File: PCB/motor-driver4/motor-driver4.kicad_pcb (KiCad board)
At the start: 2 copper layers, 100 x 100 mm, 57 parts, among them J1 Motor Power, J2 Input Logic, M1 Motor_DC, M2 Motor_DC, Q1 Q_NMOS_GDS, Q2 Q_NMOS_GDS, Q3 Q_NMOS_GDS, Q4 Q_NMOS_GDS, Q5 Q_NMOS_GDS, Q6 Q_NMOS_GDS, Q7 Q_NMOS_GDS, Q8 Q_NMOS_GDS, U1 IR2302, U2 IR2302, U3 IR2302, U4 IR2302

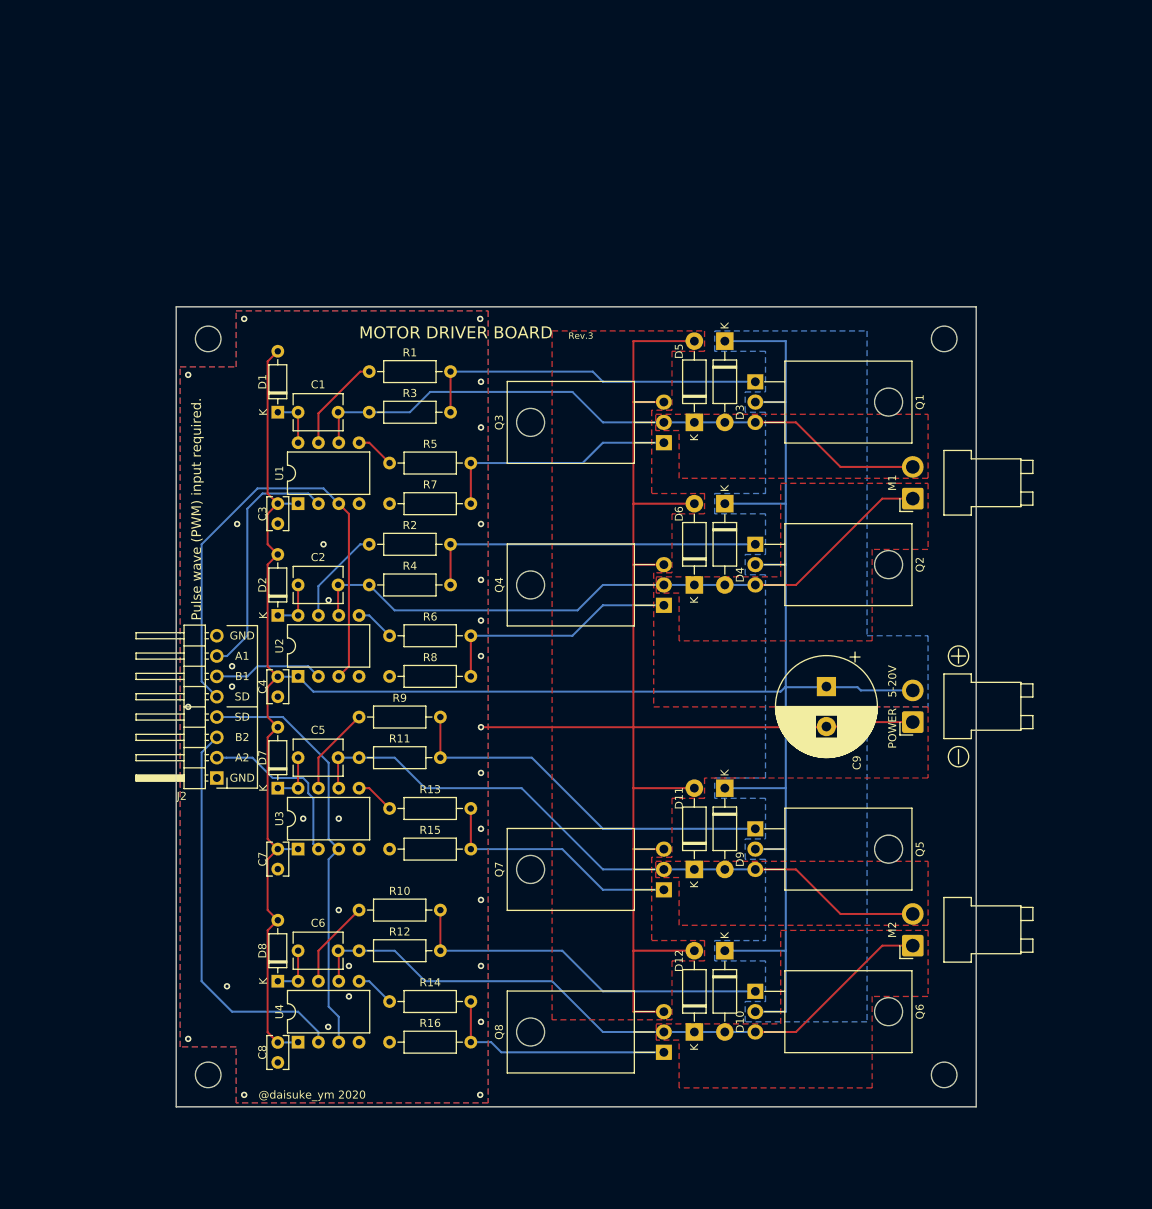
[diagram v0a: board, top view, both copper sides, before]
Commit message: ほぼ完成
git-svn-id: https://shiro-home.ddns.net/svn/project/motor-driver/trunk@12 73406841-da20-4056-b287-c5b29fcc9b8e
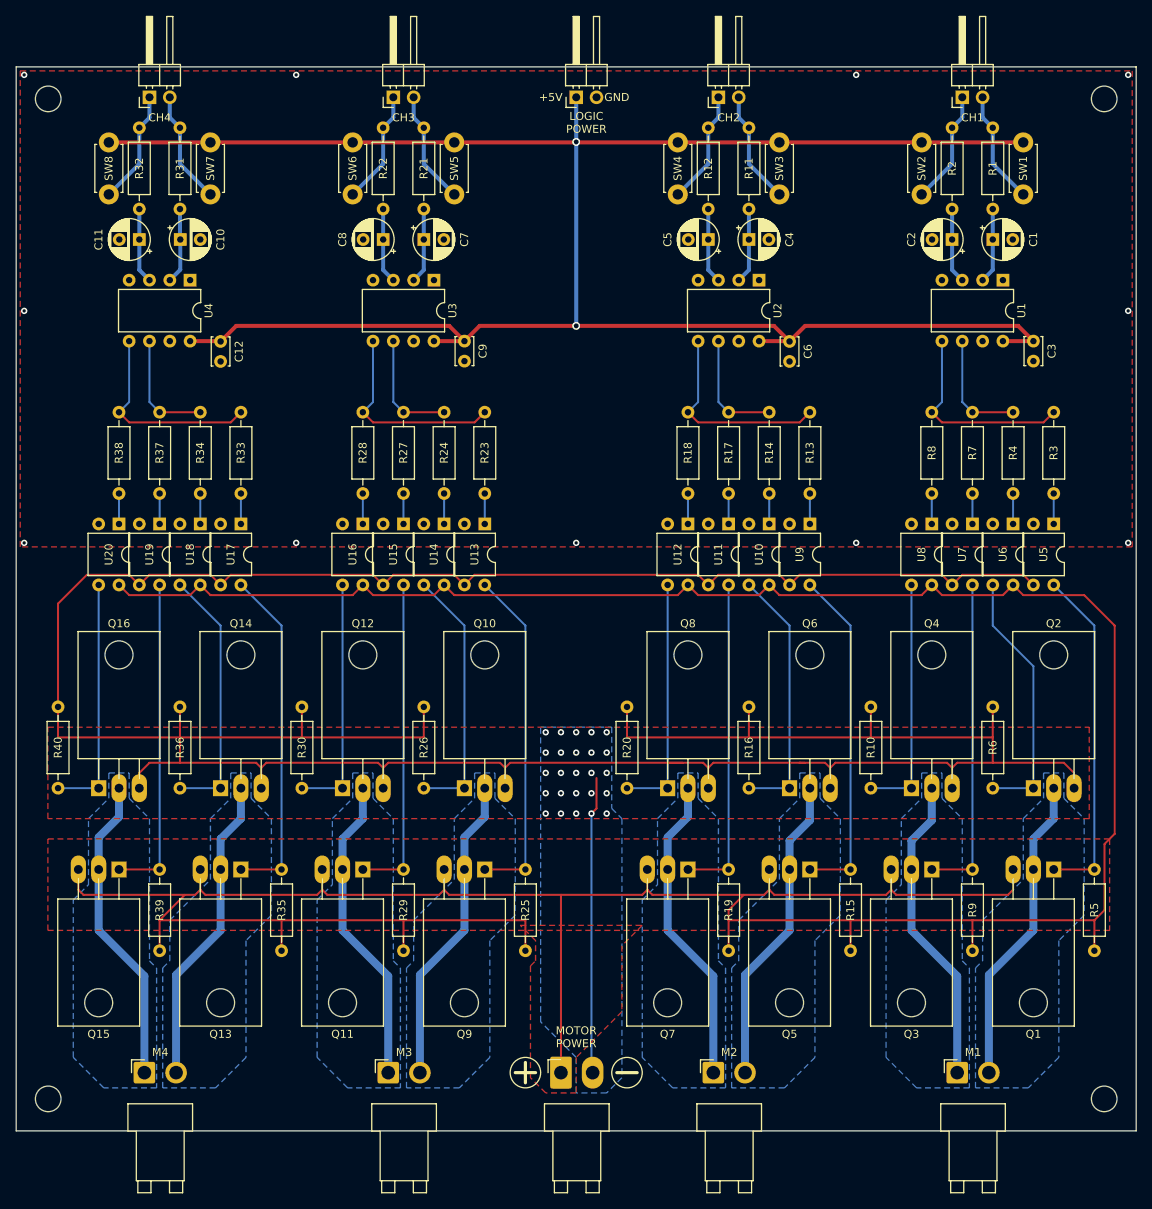
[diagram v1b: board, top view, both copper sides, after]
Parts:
- removed D1, D2, D7, D8: 1N4148, Diode_THT:D_DO-35_SOD27_P7.62mm_Horizontal
- removed D10, D11, D12, D3, D4, D5, D6, D9: 1N4007, Diode_THT:D_DO-41_SOD81_P10.16mm_Horizontal
- added C10: 10u, Capacitor_THT:CP_Radial_D5.0mm_P2.50mm, F.Cu at (100.5, 41.6)
- added C11: 10u, Capacitor_THT:CP_Radial_D5.0mm_P2.50mm, F.Cu at (95.4, 41.6)
- added C12: 0.1u, Capacitor_THT:C_Disc_D3.4mm_W2.1mm_P2.50mm, F.Cu at (105.5, 54.3)
- added J3: Input Ch1, Connector_PinHeader_2.54mm:PinHeader_1x02_P2.54mm_Horizontal, F.Cu at (198.3, 23.8)
- added J4: Input Ch2, Connector_PinHeader_2.54mm:PinHeader_1x02_P2.54mm_Horizontal, F.Cu at (167.8, 23.8)
- added J5: Input Ch3, Connector_PinHeader_2.54mm:PinHeader_1x02_P2.54mm_Horizontal, F.Cu at (127.1, 23.8)
- added J6: Input Ch4, Connector_PinHeader_2.54mm:PinHeader_1x02_P2.54mm_Horizontal, F.Cu at (96.7, 23.8)
- added M3: Motor_DC, Connector_JST:JST_VH_B2PS-VH_1x02_P3.96mm_Horizontal, F.Cu at (126.5, 145.7)
- added M4: Motor_DC, Connector_JST:JST_VH_B2PS-VH_1x02_P3.96mm_Horizontal, F.Cu at (96.0, 145.7)
- added Q10: Q_NMOS_GDS, Package_TO_SOT_THT:TO-220-3_Horizontal_TabDown, F.Cu at (136.0, 110.2)
- added Q11: Q_PMOS_GDS, Package_TO_SOT_THT:TO-220-3_Horizontal_TabDown, F.Cu at (123.3, 120.3)
- added Q12: Q_NMOS_GDS, Package_TO_SOT_THT:TO-220-3_Horizontal_TabDown, F.Cu at (120.8, 110.2)
- added Q13: Q_PMOS_GDS, Package_TO_SOT_THT:TO-220-3_Horizontal_TabDown, F.Cu at (108.1, 120.3)
- added Q14: Q_NMOS_GDS, Package_TO_SOT_THT:TO-220-3_Horizontal_TabDown, F.Cu at (105.5, 110.2)
- added Q15: Q_PMOS_GDS, Package_TO_SOT_THT:TO-220-3_Horizontal_TabDown, F.Cu at (92.8, 120.3)
- added Q16: Q_NMOS_GDS, Package_TO_SOT_THT:TO-220-3_Horizontal_TabDown, F.Cu at (90.3, 110.2)
- added Q9: Q_PMOS_GDS, Package_TO_SOT_THT:TO-220-3_Horizontal_TabDown, F.Cu at (138.6, 120.3)
- added R17: 330, Resistor_THT:R_Axial_DIN0207_L6.3mm_D2.5mm_P10.16mm_Horizontal, F.Cu at (169.1, 63.2)
- added R18: 330, Resistor_THT:R_Axial_DIN0207_L6.3mm_D2.5mm_P10.16mm_Horizontal, F.Cu at (164.0, 63.2)
- added R19: 2k2, Resistor_THT:R_Axial_DIN0207_L6.3mm_D2.5mm_P10.16mm_Horizontal, F.Cu at (169.1, 120.3)
- added R20: 2k2, Resistor_THT:R_Axial_DIN0207_L6.3mm_D2.5mm_P10.16mm_Horizontal, F.Cu at (156.3, 100.0)
- added R21: 4k7, Resistor_THT:R_Axial_DIN0207_L6.3mm_D2.5mm_P10.16mm_Horizontal, F.Cu at (130.9, 27.6)
- added R22: 4k7, Resistor_THT:R_Axial_DIN0207_L6.3mm_D2.5mm_P10.16mm_Horizontal, F.Cu at (125.9, 27.6)
- added R23: 330, Resistor_THT:R_Axial_DIN0207_L6.3mm_D2.5mm_P10.16mm_Horizontal, F.Cu at (138.6, 63.2)
- added R24: 330, Resistor_THT:R_Axial_DIN0207_L6.3mm_D2.5mm_P10.16mm_Horizontal, F.Cu at (133.5, 63.2)
- added R25: 2k2, Resistor_THT:R_Axial_DIN0207_L6.3mm_D2.5mm_P10.16mm_Horizontal, F.Cu at (143.7, 120.3)
- added R26: 2k2, Resistor_THT:R_Axial_DIN0207_L6.3mm_D2.5mm_P10.16mm_Horizontal, F.Cu at (130.9, 100.0)
- added R27: 330, Resistor_THT:R_Axial_DIN0207_L6.3mm_D2.5mm_P10.16mm_Horizontal, F.Cu at (128.4, 63.2)
- added R28: 330, Resistor_THT:R_Axial_DIN0207_L6.3mm_D2.5mm_P10.16mm_Horizontal, F.Cu at (123.3, 63.2)
- added R29: 2k2, Resistor_THT:R_Axial_DIN0207_L6.3mm_D2.5mm_P10.16mm_Horizontal, F.Cu at (128.4, 120.3)
- added R30: 2k2, Resistor_THT:R_Axial_DIN0207_L6.3mm_D2.5mm_P10.16mm_Horizontal, F.Cu at (115.7, 100.0)
- added R31: 4k7, Resistor_THT:R_Axial_DIN0207_L6.3mm_D2.5mm_P10.16mm_Horizontal, F.Cu at (100.5, 27.6)
- added R32: 4k7, Resistor_THT:R_Axial_DIN0207_L6.3mm_D2.5mm_P10.16mm_Horizontal, F.Cu at (95.4, 27.6)
- added R33: 330, Resistor_THT:R_Axial_DIN0207_L6.3mm_D2.5mm_P10.16mm_Horizontal, F.Cu at (108.1, 63.2)
- added R34: 330, Resistor_THT:R_Axial_DIN0207_L6.3mm_D2.5mm_P10.16mm_Horizontal, F.Cu at (103.0, 63.2)
- added R35: 2k2, Resistor_THT:R_Axial_DIN0207_L6.3mm_D2.5mm_P10.16mm_Horizontal, F.Cu at (113.2, 120.3)
- added R36: 2k2, Resistor_THT:R_Axial_DIN0207_L6.3mm_D2.5mm_P10.16mm_Horizontal, F.Cu at (100.5, 100.0)
- added R37: 330, Resistor_THT:R_Axial_DIN0207_L6.3mm_D2.5mm_P10.16mm_Horizontal, F.Cu at (97.9, 63.2)
- added R38: 330, Resistor_THT:R_Axial_DIN0207_L6.3mm_D2.5mm_P10.16mm_Horizontal, F.Cu at (92.8, 63.2)
- added R39: 2k2, Resistor_THT:R_Axial_DIN0207_L6.3mm_D2.5mm_P10.16mm_Horizontal, F.Cu at (97.9, 120.3)
- added R40: 2k2, Resistor_THT:R_Axial_DIN0207_L6.3mm_D2.5mm_P10.16mm_Horizontal, F.Cu at (85.2, 100.0)
- added SW1: SW_Push, MyLib:TactSW_TVBP06_3.5x6.0-ThroughHole, F.Cu at (205.9, 32.7)
- added SW2: SW_Push, MyLib:TactSW_TVBP06_3.5x6.0-ThroughHole, F.Cu at (193.2, 32.7)
- added SW3: SW_Push, MyLib:TactSW_TVBP06_3.5x6.0-ThroughHole, F.Cu at (175.4, 32.7)
- added SW4: SW_Push, MyLib:TactSW_TVBP06_3.5x6.0-ThroughHole, F.Cu at (162.7, 32.7)
- added SW5: SW_Push, MyLib:TactSW_TVBP06_3.5x6.0-ThroughHole, F.Cu at (134.8, 32.7)
- added SW6: SW_Push, MyLib:TactSW_TVBP06_3.5x6.0-ThroughHole, F.Cu at (122.1, 32.7)
- added SW7: SW_Push, MyLib:TactSW_TVBP06_3.5x6.0-ThroughHole, F.Cu at (104.3, 32.7)
- added SW8: SW_Push, MyLib:TactSW_TVBP06_3.5x6.0-ThroughHole, F.Cu at (91.6, 32.7)
- added U10: TLP785, Package_DIP:DIP-4_W7.62mm, F.Cu at (174.1, 77.1)
- added U11: TLP785, Package_DIP:DIP-4_W7.62mm, F.Cu at (169.1, 77.1)
- added U12: TLP785, Package_DIP:DIP-4_W7.62mm, F.Cu at (164.0, 77.1)
- added U13: TLP785, Package_DIP:DIP-4_W7.62mm, F.Cu at (138.6, 77.1)
- added U14: TLP785, Package_DIP:DIP-4_W7.62mm, F.Cu at (133.5, 77.1)
- added U15: TLP785, Package_DIP:DIP-4_W7.62mm, F.Cu at (128.4, 77.1)
- added U16: TLP785, Package_DIP:DIP-4_W7.62mm, F.Cu at (123.3, 77.1)
- added U17: TLP785, Package_DIP:DIP-4_W7.62mm, F.Cu at (108.1, 77.1)
- added U18: TLP785, Package_DIP:DIP-4_W7.62mm, F.Cu at (103.0, 77.1)
- added U19: TLP785, Package_DIP:DIP-4_W7.62mm, F.Cu at (97.9, 77.1)
- added U20: TLP785, Package_DIP:DIP-4_W7.62mm, F.Cu at (92.8, 77.1)
- added U5: TLP785, Package_DIP:DIP-4_W7.62mm, F.Cu at (209.7, 77.1)
- added U6: TLP785, Package_DIP:DIP-4_W7.62mm, F.Cu at (204.6, 77.1)
- added U7: TLP785, Package_DIP:DIP-4_W7.62mm, F.Cu at (199.5, 77.1)
- added U8: TLP785, Package_DIP:DIP-4_W7.62mm, F.Cu at (194.4, 77.1)
- added U9: TLP785, Package_DIP:DIP-4_W7.62mm, F.Cu at (179.2, 77.1)
- C1, C2, C5: footprint Capacitor_THT:C_Disc_D6.0mm_W4.4mm_P5.00mm -> Capacitor_THT:CP_Radial_D5.0mm_P2.50mm
- C3: footprint Capacitor_THT:C_Rect_L4.0mm_W2.5mm_P2.50mm -> Capacitor_THT:C_Disc_D3.4mm_W2.1mm_P2.50mm
- C4, C7, C8: value 0.1u -> 10u; footprint Capacitor_THT:C_Rect_L4.0mm_W2.5mm_P2.50mm -> Capacitor_THT:CP_Radial_D5.0mm_P2.50mm
- C6: value 10u -> 0.1u; footprint Capacitor_THT:C_Disc_D6.0mm_W4.4mm_P5.00mm -> Capacitor_THT:C_Disc_D3.4mm_W2.1mm_P2.50mm
- C9: value 470u 50V -> 0.1u; footprint Capacitor_THT:CP_Radial_D12.5mm_P5.00mm -> Capacitor_THT:C_Disc_D3.4mm_W2.1mm_P2.50mm
- J2: value Input Logic -> Logic Power; footprint Connector_PinHeader_2.54mm:PinHeader_1x08_P2.54mm_Horizontal -> Connector_PinHeader_2.54mm:PinHeader_1x02_P2.54mm_Horizontal
- Q1, Q3, Q5, Q7: value Q_NMOS_GDS -> Q_PMOS_GDS
- R1, R11, R12, R2: value 47k -> 4k7
- R10, R15, R16, R5, R6, R9: value 47k -> 2k2
- R13, R14, R3, R4, R7, R8: value 47k -> 330
- U1, U2, U3, U4: value IR2302 -> ATtiny85-20PU
- moved MH1 165.6 mm to (216.0, 24.0)
- moved MH3 115.9 mm to (84.0, 24.0)
- moved R12 111.7 mm to (166.5, 27.6), turned to 270 degrees
- moved R5 101.7 mm to (214.8, 120.3), turned to 270 degrees
- moved C8 101.2 mm to (125.9, 41.6), turned to 180 degrees
- moved C6 97.8 mm to (176.7, 54.3), turned to 270 degrees
- moved MH4 97.1 mm to (84.0, 149.0)
- moved C3 96.6 mm to (207.2, 54.3)
- moved J2 96.2 mm to (150.0, 23.8), turned to 90 degrees
- moved U4 96.2 mm to (101.7, 46.7), turned to 270 degrees
- moved R11 92.6 mm to (171.6, 27.6), turned to 270 degrees
- moved C2 92.5 mm to (197.0, 41.6), turned to 180 degrees
- moved U1 92.4 mm to (203.3, 46.7), turned to 270 degrees
- moved R2 89.6 mm to (197.0, 27.6), turned to 270 degrees
- moved C1 89.5 mm to (202.1, 41.6)
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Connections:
- C1 pad 1: Net-(C1-Pad1) -> /IN1AA
- C1 pad 2: Net-(C1-Pad2) -> GND
- C2 pad 1: Net-(C2-Pad1) -> /IN1BA
- C2 pad 2: Net-(C2-Pad2) -> GND
- C3 pad 1: +BATT -> +5V
- C3 pad 2: GNDPWR -> GND
- C4 pad 1: +BATT -> /IN2AA
- C4 pad 2: GNDPWR -> GND
- C5 pad 1: Net-(C5-Pad1) -> /IN2BA
- C5 pad 2: Net-(C5-Pad2) -> GND
- C6 pad 1: Net-(C6-Pad1) -> +5V
- C6 pad 2: Net-(C6-Pad2) -> GND
- C7 pad 1: +BATT -> /IN3AA
- C7 pad 2: GNDPWR -> GND
- C8 pad 1: +BATT -> /IN3BA
- C8 pad 2: GNDPWR -> GND
- C9 pad 1: +BATT -> +5V
- C9 pad 2: GNDPWR -> GND
- J1 pad 1: GNDPWR -> +BATT
- J1 pad 2: +BATT -> GNDPWR
- J2 pad 1: GNDPWR -> +5V
- J2 pad 2: /IN_A2 -> GND
- M1 pad 1: Net-(C2-Pad2) -> Net-(M1-Pad1)
- M1 pad 2: Net-(C1-Pad2) -> Net-(M1-Pad2)
- M2 pad 1: Net-(C6-Pad2) -> Net-(M2-Pad1)
- M2 pad 2: Net-(C5-Pad2) -> Net-(M2-Pad2)
- Q1 pad 2: +BATT -> Net-(M1-Pad2)
- Q1 pad 3: Net-(C1-Pad2) -> +BATT
- Q2 pad 2: +BATT -> Net-(M1-Pad2)
- Q2 pad 3: Net-(C2-Pad2) -> GNDPWR
- Q3 pad 2: Net-(C1-Pad2) -> Net-(M1-Pad1)
- Q3 pad 3: GNDPWR -> +BATT
- Q4 pad 2: Net-(C2-Pad2) -> Net-(M1-Pad1)
- Q5 pad 2: +BATT -> Net-(M2-Pad2)
- Q5 pad 3: Net-(C5-Pad2) -> +BATT
- Q6 pad 2: +BATT -> Net-(M2-Pad2)
- Q6 pad 3: Net-(C6-Pad2) -> GNDPWR
- Q7 pad 2: Net-(C5-Pad2) -> Net-(M2-Pad1)
- Q7 pad 3: GNDPWR -> +BATT
- Q8 pad 2: Net-(C6-Pad2) -> Net-(M2-Pad1)
- R1 pad 1: Net-(R1-Pad1) -> /IN1A
- R1 pad 2: Net-(Q1-Pad1) -> /IN1AA
- R10 pad 1: Net-(R10-Pad1) -> GNDPWR
- R10 pad 2: Net-(Q6-Pad1) -> Net-(Q4-Pad1)
- R11 pad 1: Net-(C5-Pad2) -> /IN2A
- R11 pad 2: Net-(Q5-Pad1) -> /IN2AA
- R12 pad 1: Net-(C6-Pad2) -> /IN2B
- R12 pad 2: Net-(Q6-Pad1) -> /IN2BA
- R13 pad 1: Net-(R13-Pad1) -> /PC2A
- R13 pad 2: Net-(Q7-Pad1) -> Net-(R13-Pad2)
- R14 pad 1: Net-(R14-Pad1) -> /PC2B
- R14 pad 2: Net-(Q8-Pad1) -> Net-(R14-Pad2)
- R15 pad 1: GNDPWR -> Net-(Q5-Pad1)
- R15 pad 2: Net-(Q7-Pad1) -> +BATT
- R16 pad 2: Net-(Q8-Pad1) -> Net-(Q6-Pad1)
- R2 pad 1: Net-(R2-Pad1) -> /IN1B
- R2 pad 2: Net-(Q2-Pad1) -> /IN1BA
- R3 pad 1: Net-(C1-Pad2) -> /PC1A
- R3 pad 2: Net-(Q1-Pad1) -> Net-(R3-Pad2)
- R4 pad 1: Net-(C2-Pad2) -> /PC1B
- R4 pad 2: Net-(Q2-Pad1) -> Net-(R4-Pad2)
- R5 pad 1: Net-(R5-Pad1) -> Net-(Q1-Pad1)
- R5 pad 2: Net-(Q3-Pad1) -> +BATT
- R6 pad 1: Net-(R6-Pad1) -> GNDPWR
- R6 pad 2: Net-(Q4-Pad1) -> Net-(Q2-Pad1)
- R7 pad 1: GNDPWR -> /PC1B
- R7 pad 2: Net-(Q3-Pad1) -> Net-(R7-Pad2)
- R8 pad 1: GNDPWR -> /PC1A
- R8 pad 2: Net-(Q4-Pad1) -> Net-(R8-Pad2)
- R9 pad 1: Net-(R9-Pad1) -> Net-(Q3-Pad1)
- R9 pad 2: Net-(Q5-Pad1) -> +BATT
- U1 pad 1: +BATT -> Net-(U1-Pad1)
- U1 pad 2: /IN_A1 -> /IN1AA
- U1 pad 3: /IN_SD1 -> /IN1BA
- U1 pad 4: GNDPWR -> GND
- U1 pad 5: Net-(R5-Pad1) -> /PC1A
- U1 pad 6: Net-(C1-Pad2) -> /PC1B
- U1 pad 7: Net-(R1-Pad1) -> Net-(U1-Pad7)
- U1 pad 8: Net-(C1-Pad1) -> +5V
- U2 pad 1: +BATT -> Net-(U2-Pad1)
- U2 pad 2: /IN_B1 -> /IN2AA
- U2 pad 3: /IN_SD1 -> /IN2BA
- U2 pad 4: GNDPWR -> GND
- U2 pad 5: Net-(R6-Pad1) -> /PC2A
- U2 pad 6: Net-(C2-Pad2) -> /PC2B
- U2 pad 7: Net-(R2-Pad1) -> Net-(U2-Pad7)
- U2 pad 8: Net-(C2-Pad1) -> +5V
- U3 pad 1: +BATT -> Net-(U3-Pad1)
- U3 pad 2: /IN_A2 -> /IN3AA
- U3 pad 3: /IN_SD2 -> /IN3BA
- U3 pad 4: GNDPWR -> GND
- U3 pad 5: Net-(R13-Pad1) -> /PC3A
- U3 pad 6: Net-(C5-Pad2) -> /PC3B
- U3 pad 7: Net-(R9-Pad1) -> Net-(U3-Pad7)
- U3 pad 8: Net-(C5-Pad1) -> +5V
- U4 pad 1: +BATT -> Net-(U4-Pad1)
- U4 pad 2: /IN_B2 -> /IN4AA
- U4 pad 3: /IN_SD2 -> /IN4BA
- U4 pad 4: GNDPWR -> GND
- U4 pad 5: Net-(R14-Pad1) -> /PC4A
- U4 pad 6: Net-(C6-Pad2) -> /PC4B
- U4 pad 7: Net-(R10-Pad1) -> Net-(U4-Pad7)
- U4 pad 8: Net-(C6-Pad1) -> +5V
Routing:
- net GNDPWR: track 183.8 -> 452.3 mm, vias 31 -> 25
- net +5V: track 0.00 -> 264.6 mm, vias 0 -> 2
- net +BATT: track 311.6 -> 465.3 mm
- net Net-(C6-Pad2): track 84.4 -> 0.00 mm
- net Net-(C5-Pad2): track 83.8 -> 0.00 mm
- net Net-(C2-Pad2): track 82.8 -> 0.00 mm
- net Net-(C1-Pad2): track 80.6 -> 0.00 mm
- net /IN_SD1: track 63.3 -> 0.00 mm
- net /IN_SD2: track 52.8 -> 0.00 mm
- net /IN_B2: track 49.8 -> 0.00 mm
- net Net-(Q9-Pad1): track 0.00 -> 42.7 mm
- net Net-(Q13-Pad1): track 0.00 -> 42.7 mm
- net Net-(Q15-Pad1): track 0.00 -> 40.6 mm
- net Net-(Q11-Pad1): track 0.00 -> 40.6 mm
- net Net-(M4-Pad1): track 0.00 -> 39.0 mm
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- added copper zone on F.Cu, net +BATT
- added copper zone on F.Cu, net GND
- added copper zone on B.Cu, net Net-(M1-Pad1)
- added copper zone on B.Cu, net Net-(M1-Pad2)
- added copper zone on B.Cu, net Net-(M2-Pad1)
- added copper zone on B.Cu, net Net-(M2-Pad2)
- added copper zone on B.Cu, net Net-(M3-Pad1)
- added copper zone on B.Cu, net Net-(M3-Pad2)
- added copper zone on B.Cu, net Net-(M4-Pad1)
- added copper zone on B.Cu, net Net-(M4-Pad2)
- removed copper zone on B.Cu, net +BATT
- removed copper zone on F.Cu, net Net-(C1-Pad2)
- removed copper zone on F.Cu, net Net-(C2-Pad2)
- removed copper zone on F.Cu, net Net-(C5-Pad2)
- removed copper zone on F.Cu, net Net-(C6-Pad2)
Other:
- board size 100 x 100 mm -> 140 x 133 mm
- net class Input added: clearance 0.3, trace_width 0.5, via_dia 1, via_drill 0.6
- board text added: "+5V"
- board text added: "CH1"
- board text added: "CH2"
- board text added: "CH3"
- board text added: "CH4"
- board text added: "LOGIC POWER"
- board text added: "MOTOR POWER"
- board text removed: "@daisuke_ym 2020"
- board text removed: "A1"
- board text removed: "A2"
- board text removed: "B1"
- board text removed: "B2"
- board text removed: "MOTOR DRIVER BOARD"
- board text removed: "POWER 5-20V"
- board text removed: "Pulse wave (PWM) input required."
- board text removed: "Rev.3"
- board text removed: "SD"
